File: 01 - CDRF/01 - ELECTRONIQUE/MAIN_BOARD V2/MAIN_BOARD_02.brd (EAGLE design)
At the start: 85 x 85 mm, 40 parts, among them J5 CONN_05, J6 CONN_05, J8 CONN_05, U1 74HC165SO-16

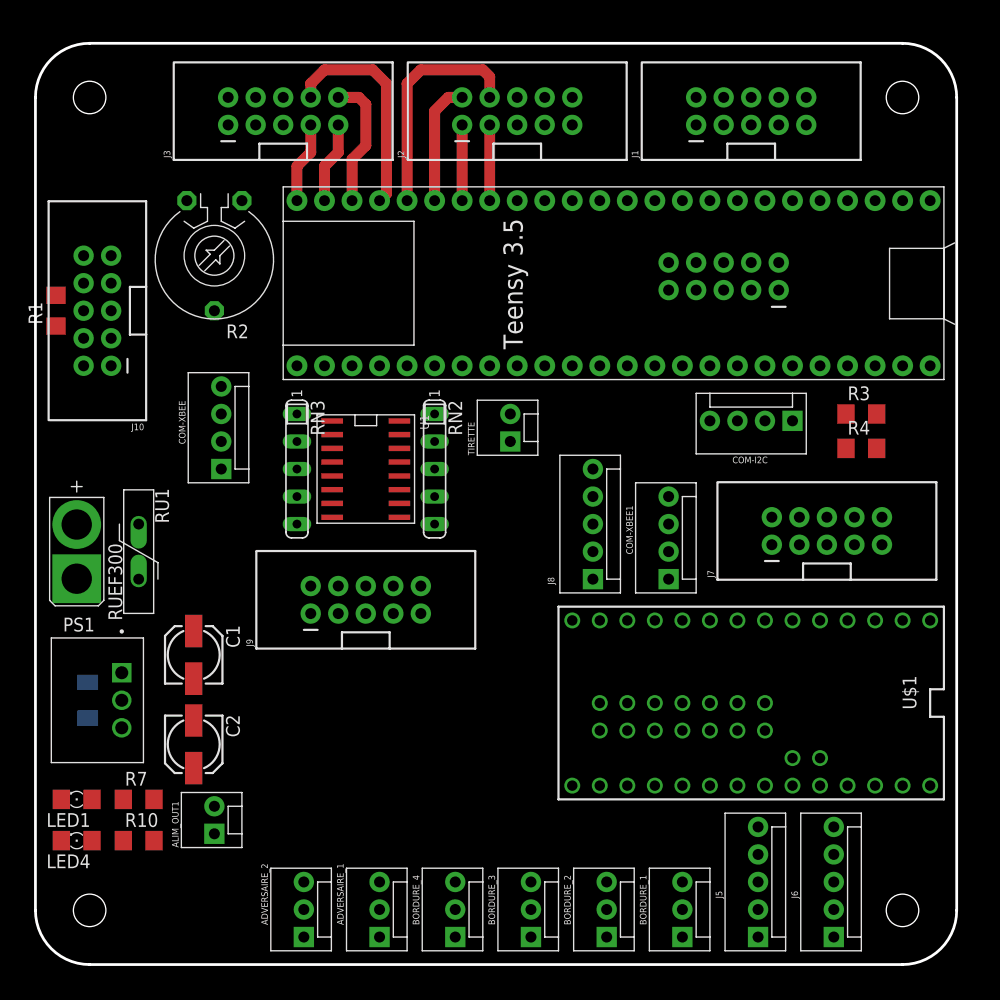
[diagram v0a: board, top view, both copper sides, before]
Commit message: Update PCB
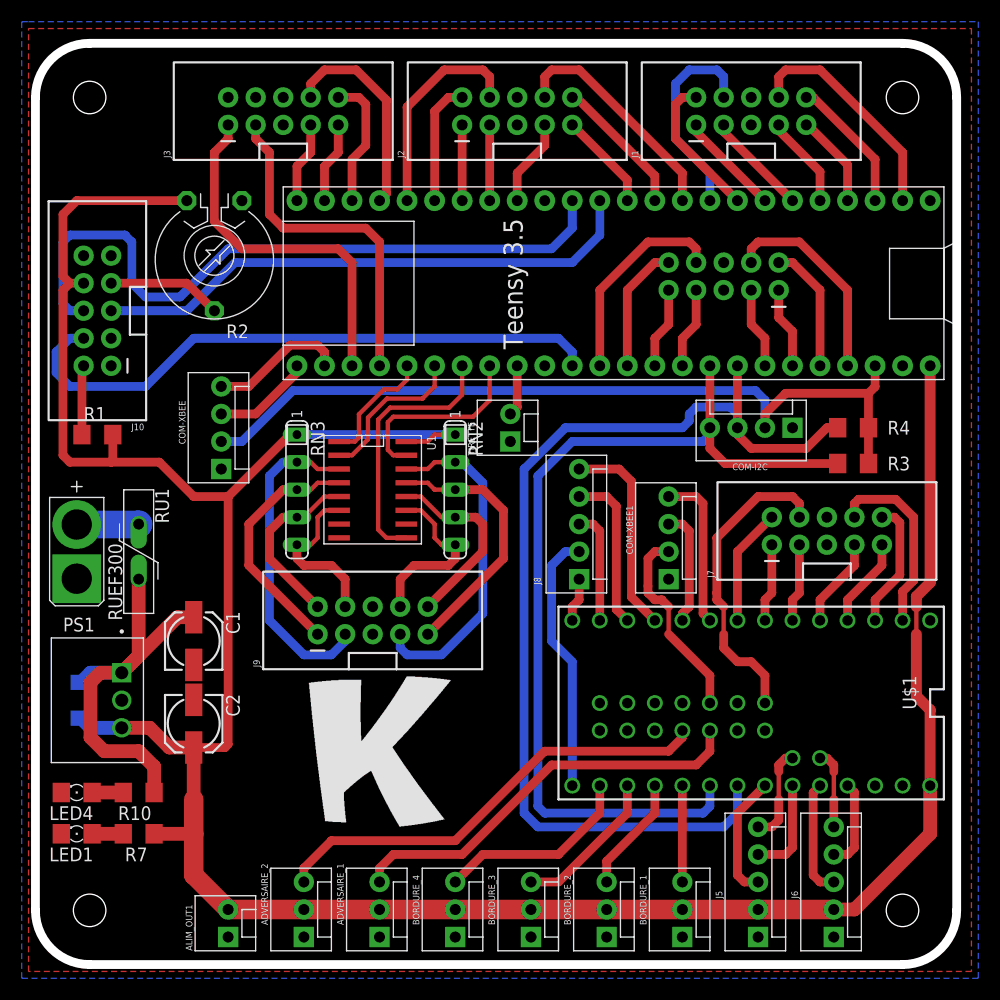
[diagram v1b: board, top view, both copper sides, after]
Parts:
- added U$3, U$4: LOGO_K, KARIBOUS:LOGO_KARIBOU
- moved R1 12.0 mm to (5.71, 48.9), turned to 0 degrees
- moved ALIM_OUT1 9.61 mm to (17.8, 2.54)
- moved R3 4.64 mm to (75.4, 46.2)
- moved LED4 4.45 mm to (3.81, 15.9)
- moved R10 4.45 mm to (9.53, 15.9)
- moved LED1 3.18 mm to (3.81, 12.1)
- moved R7 3.18 mm to (9.53, 12.1)
- moved RN2 2.69 mm to (38.7, 43.8)
- moved R4 2.05 mm to (75.4, 49.5)
- moved J9 2.01 mm to (31.1, 31.8)
- moved U1 2.01 mm to (31.1, 43.8)
- moved C2 1.91 mm to (14.6, 22.2)
- moved RN3 1.91 mm to (24.1, 43.8)
- moved J8 1.27 mm to (50.2, 35.6)
- moved C1 1.27 mm to (14.6, 29.8)
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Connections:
- net MISO_DRIVER: now also J8.1; no longer J8.2
- net SCK_DRIVER: now also J8.2; no longer J8.1
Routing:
- net +5V: track 0.00 -> 253.0 mm
- net SCL: track 0.00 -> 95.9 mm
- net SDA: track 0.00 -> 86.9 mm
- net +3V3/1: track 0.00 -> 75.9 mm
- net MISO: track 0.00 -> 64.9 mm
- net SCK: track 0.00 -> 56.8 mm
- net MOSI: track 0.00 -> 51.2 mm
- net IO-ADVERSAIRE2: track 0.00 -> 41.8 mm
- net VIN/BATT: track 0.00 -> 39.9 mm
- net IO-ADVERSAIRE1: track 0.00 -> 38.1 mm
- net CON3-7: track 0.00 -> 33.2 mm
- net CON3-8: track 0.00 -> 31.4 mm
- net D3: track 0.00 -> 30.9 mm
- net D4: track 0.00 -> 30.0 mm
- net M0: track 0.00 -> 28.6 mm
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- added copper zone on layer 1, net GND
- added copper zone on layer 16, net GND
